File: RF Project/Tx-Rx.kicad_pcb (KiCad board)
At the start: 2 copper layers, 30 x 55 mm, 26 parts, among them J1 CONN_Right, J2 CONN_Left, U1 CC2500RGPR, U2 U.FL_male

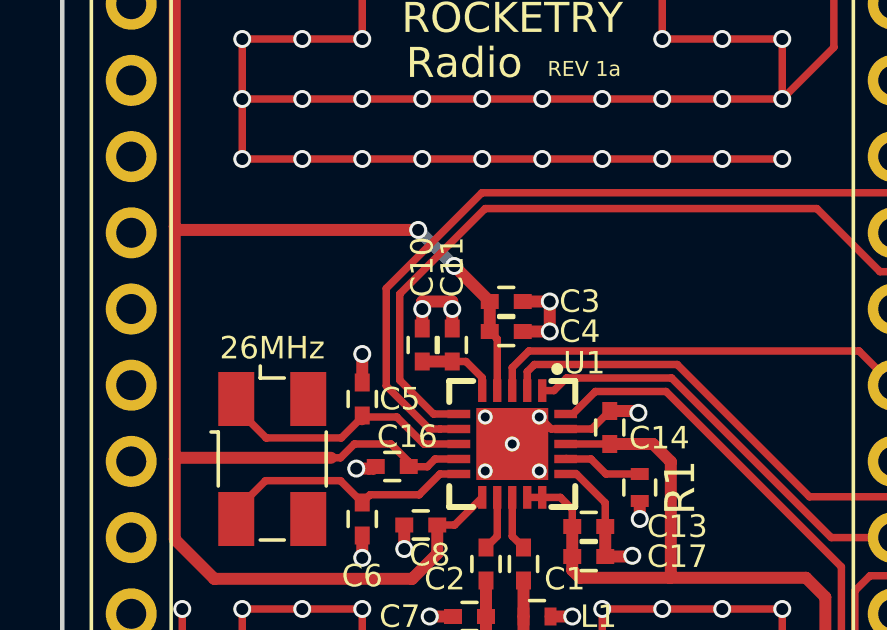
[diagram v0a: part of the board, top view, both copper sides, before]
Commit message: Fixed my poor attempt to move stuff :(
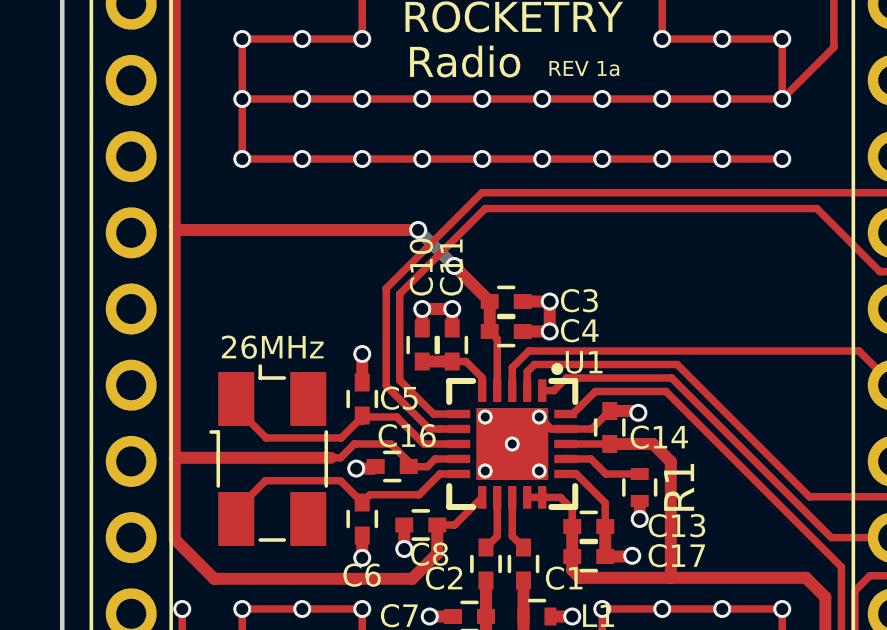
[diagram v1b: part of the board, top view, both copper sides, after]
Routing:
- net PWR_GND: track 273.5 -> 273.0 mm
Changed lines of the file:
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@@
   (segment (start 99.25 103.75) (end 99.5 104) (width 0.25) (layer F.Cu) (net 7))
   (segment (start 99.5 104) (end 99.5 105.72) (width 0.25) (layer F.Cu) (net 7))
+  (segment (start 98 103) (end 98 103.65) (width 0.4) (layer F.Cu) (net 8))
+  (segment (start 97 103) (end 98 103) (width 0.4) (layer F.Cu) (net 8))
+  (via (at 98 103) (size 0.6) (drill 0.4) (layers F.Cu B.Cu) (net 8))
+  (segment (start 97 103.65) (end 97 103) (width 0.4) (layer F.Cu) (net 8))
+  (via (at 97 103) (size 0.6) (drill 0.4) (layers F.Cu B.Cu) (net 8))
   (segment (start 96.4 110.2) (end 96.4 111) (width 0.4) (layer F.Cu) (net 8))
   (via (at 96.4 111) (size 0.6) (drill 0.4) (layers F.Cu B.Cu) (net 8))
@@
   (segment (start 95 105.45) (end 95 104.5) (width 0.4) (layer F.Cu) (net 8))
   (via (at 95 104.5) (size 0.6) (drill 0.4) (layers F.Cu B.Cu) (net 8))
-  (segment (start 98 102.75) (end 98 103.65) (width 0.4) (layer F.Cu) (net 8))
-  (segment (start 97 102.75) (end 98 102.75) (width 0.4) (layer F.Cu) (net 8))
-  (segment (start 97 103.65) (end 97 102.75) (width 0.4) (layer F.Cu) (net 8))
   (via (at 98.125 120.5) (size 0.6) (drill 0.4) (layers F.Cu B.Cu) (net 8))
   (segment (start 98.9 117) (end 98.125 117) (width 0.25) (layer F.Cu) (net 8))
@@
   (segment (start 101.775 123.6) (end 102.625 122.75) (width 0.25) (layer F.Cu) (net 8))
   (via (at 102.625 122.75) (size 0.6) (drill 0.4) (layers F.Cu B.Cu) (net 8))
-  (via (at 98 103) (size 0.6) (drill 0.4) (layers F.Cu B.Cu) (net 8))
-  (via (at 97 103) (size 0.6) (drill 0.4) (layers F.Cu B.Cu) (net 8))
   (segment (start 99.125 115.75) (end 99.441876 115.75) (width 0.4) (layer F.Cu) (net 9))
   (segment (start 99.441876 115.75) (end 99.44203 115.750154) (width 0.4) (layer F.Cu) (net 9))
